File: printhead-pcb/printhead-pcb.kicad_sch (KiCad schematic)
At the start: 22 parts, among them Q1 2N3819, Q2 BSS138, Q3 2N3819, Q4 BSS138, U1 NE555D, U2 NE555D

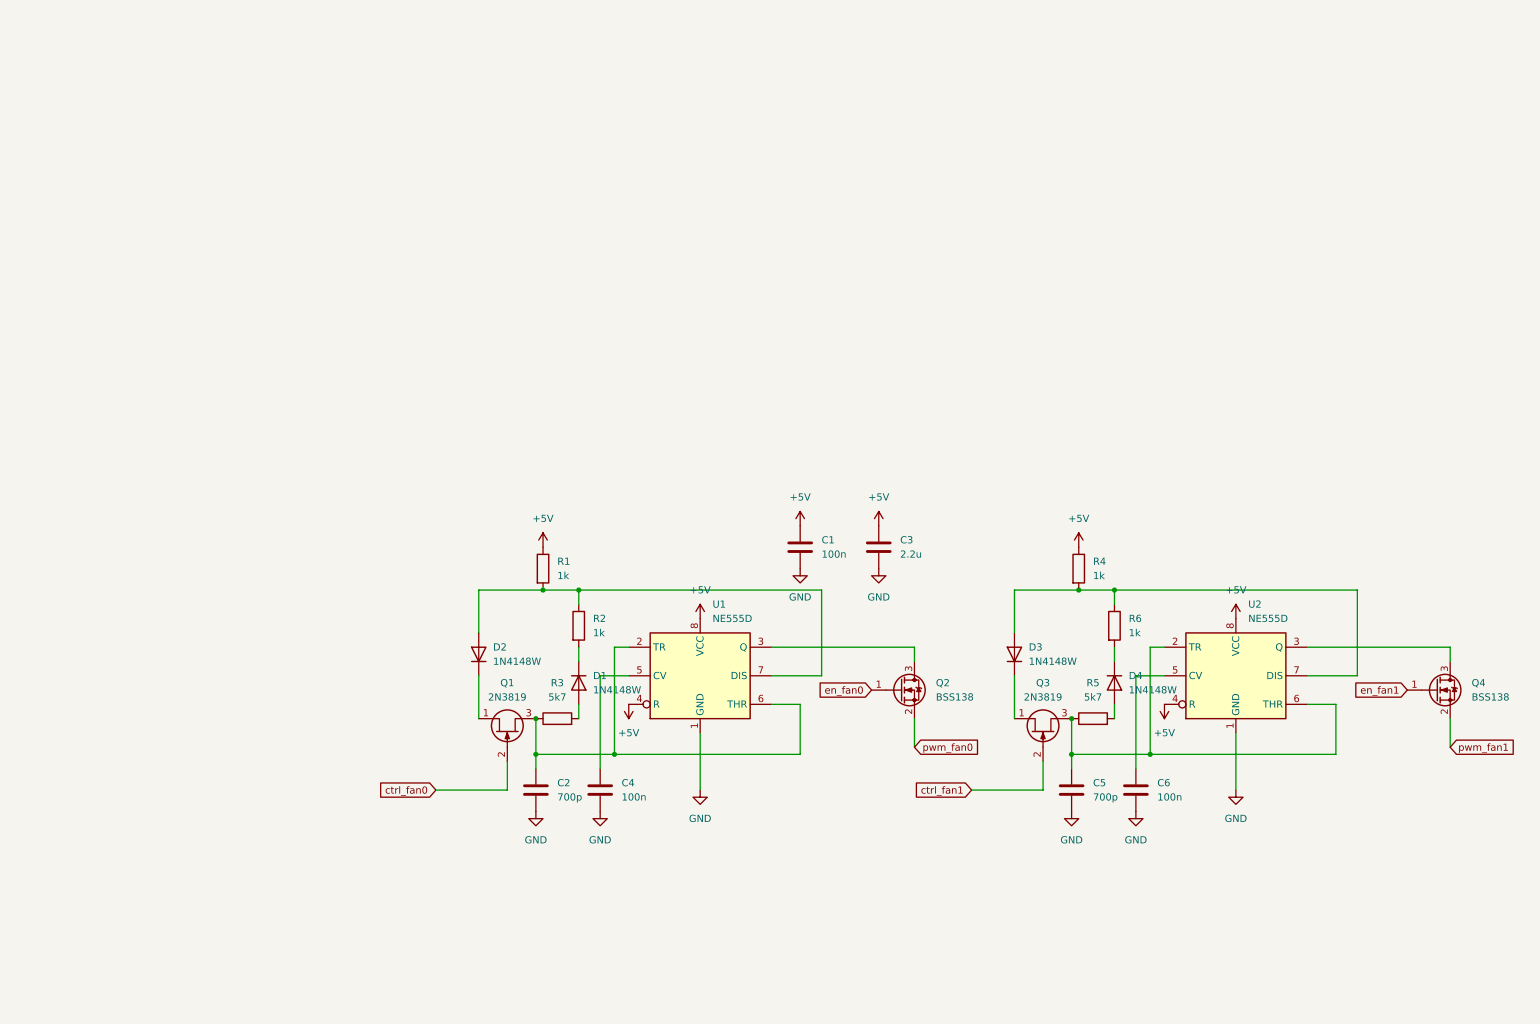
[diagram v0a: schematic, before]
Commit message: power fans, sensors
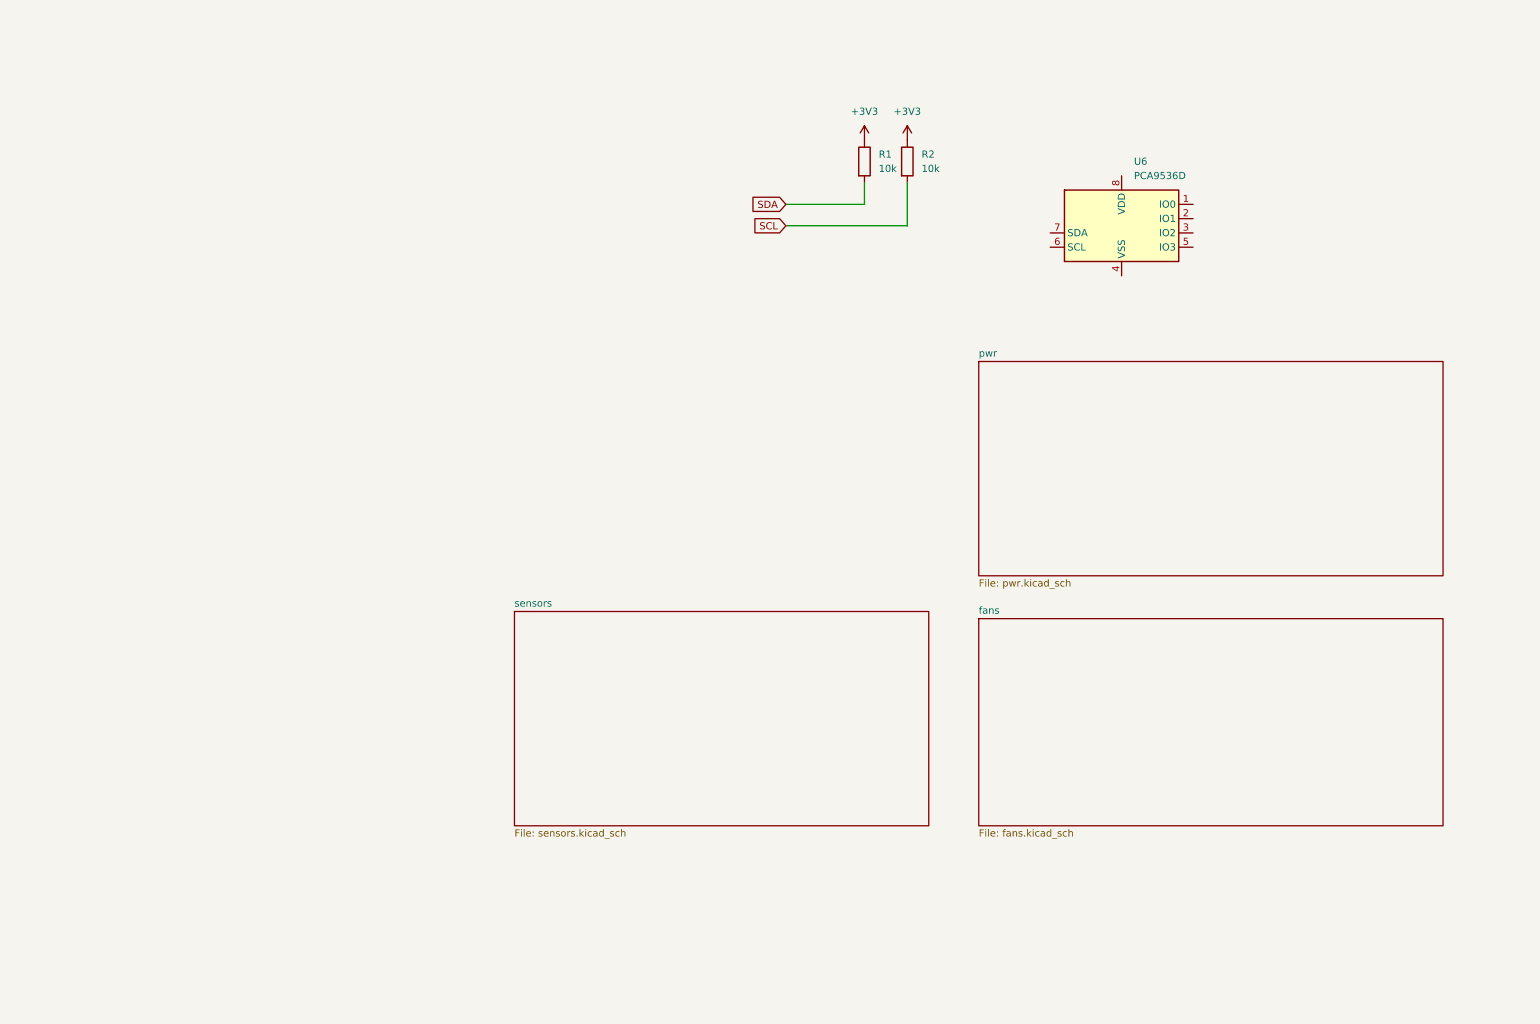
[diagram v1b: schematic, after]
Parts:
- removed C1, C4, C6: 100n, Capacitor_SMD:C_0603_1608Metric, symbol Device:C
- removed C2, C5: 700p, Capacitor_SMD:C_0603_1608Metric, symbol Device:C
- removed C3: 2.2u, Capacitor_SMD:C_1210_3225Metric, symbol Device:C
- removed D1, D2, D3, D4: 1N4148W, Diode_SMD:D_SOD-123, symbol Diode:1N4148W
- removed Q1, Q3: 2N3819, Package_DIP:DIP-8_W7.62mm_SMDSocket_SmallPads, symbol Transistor_FET:2N3819
- removed Q2, Q4: BSS138, Package_TO_SOT_SMD:SOT-23, symbol Transistor_FET:BSS138
- removed R3, R5: 5k7, Resistor_SMD:R_0603_1608Metric, symbol Device:R
- removed R4, R6: 1k, Resistor_SMD:R_0603_1608Metric, symbol Device:R
- removed U1, U2: NE555D, Package_SO:SOIC-8_3.9x4.9mm_P1.27mm, symbol Timer:NE555D
- added U6: PCA9536D, Package_SO:SOIC-8_3.9x4.9mm_P1.27mm, symbol Interface_Expansion:PCA9536D
- R1, R2: value 1k -> 10k; footprint Resistor_SMD:R_0603_1608Metric -> (none)
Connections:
- net +5V is gone; now on net +3V3: R1.1
- net +3V3: now reaches R2.1
- net +3V3: no longer R1.2
- net SCL: now reaches R2.2
- new net SDA: R1.2
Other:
- added sheet fans (fans.kicad_sch)
- added sheet pwr (pwr.kicad_sch)
- added sheet sensors (sensors.kicad_sch)

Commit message: circuit finished?
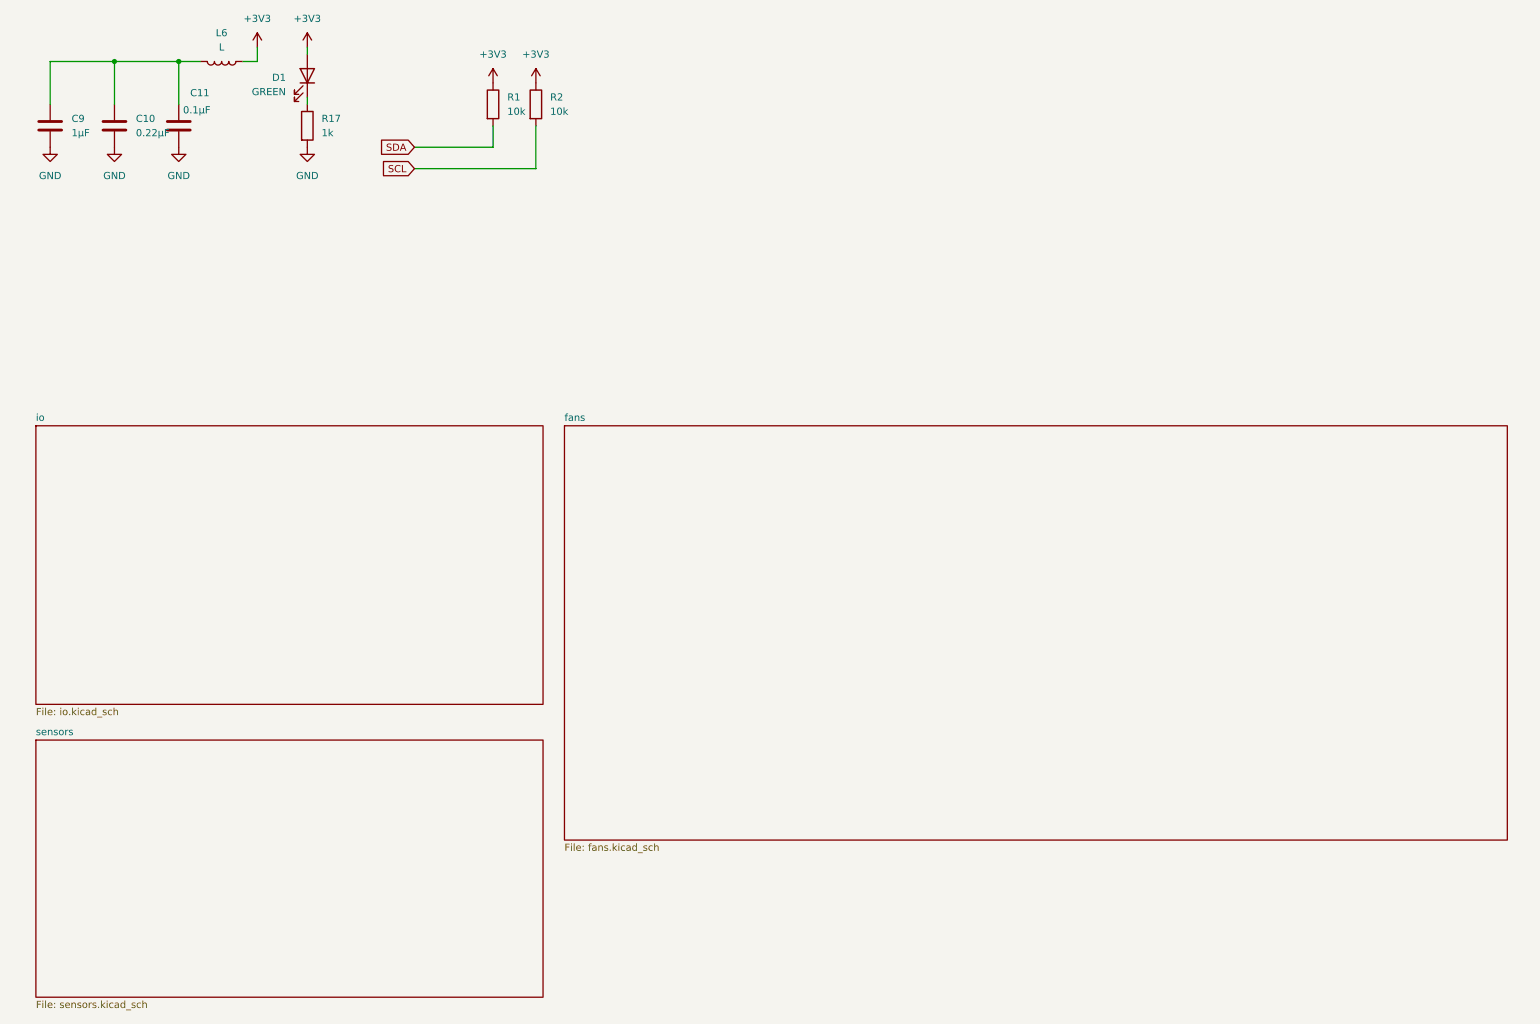
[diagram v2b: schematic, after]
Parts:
- removed U6: PCA9536D, Package_SO:SOIC-8_3.9x4.9mm_P1.27mm, symbol Interface_Expansion:PCA9536D
- added C10: 0.22µF, Capacitor_SMD:C_0402_1005Metric, symbol Device:C
- added C11: 0.1µF, Capacitor_SMD:C_0402_1005Metric, symbol Device:C
- added C9: 1µF, Capacitor_SMD:C_0402_1005Metric, symbol Device:C
- added D1: GREEN, LED_SMD:LED_0805_2012Metric, symbol Device:LED
- added L6: L, Inductor_SMD:L_0402_1005Metric, symbol Device:L
- added R17: 1k, Resistor_SMD:R_0402_1005Metric, symbol Device:R
- R1, R2: footprint (none) -> Resistor_SMD:R_0402_1005Metric
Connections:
- net +3V3: now also D1.2 (A), L6.1
- new net: D1.1 (K), R17.1
- new net: C10.1, C11.1, C9.1, L6.2
- new net GND: C10.2, C11.2, C9.2, R17.2
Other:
- removed sheet pwr
- added sheet io (io.kicad_sch)
- title: (none) -> Printhead PCB
- moved on the sheet: R1, R2

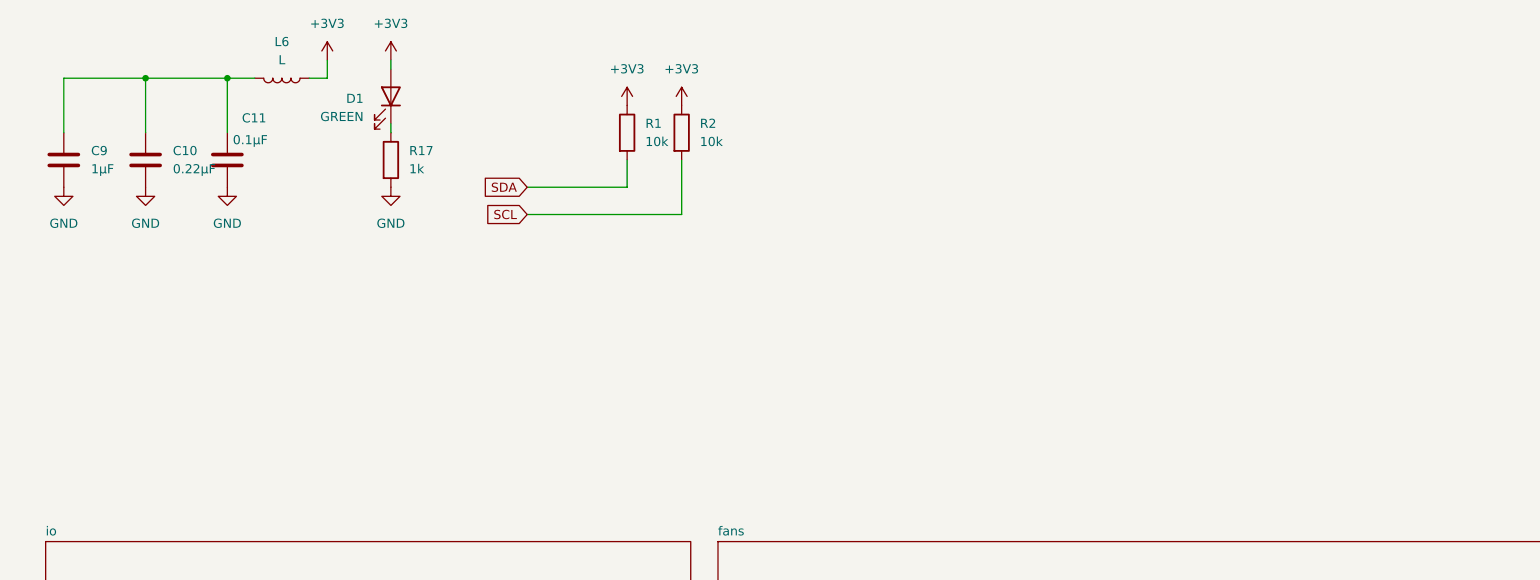
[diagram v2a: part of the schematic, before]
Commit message: layout
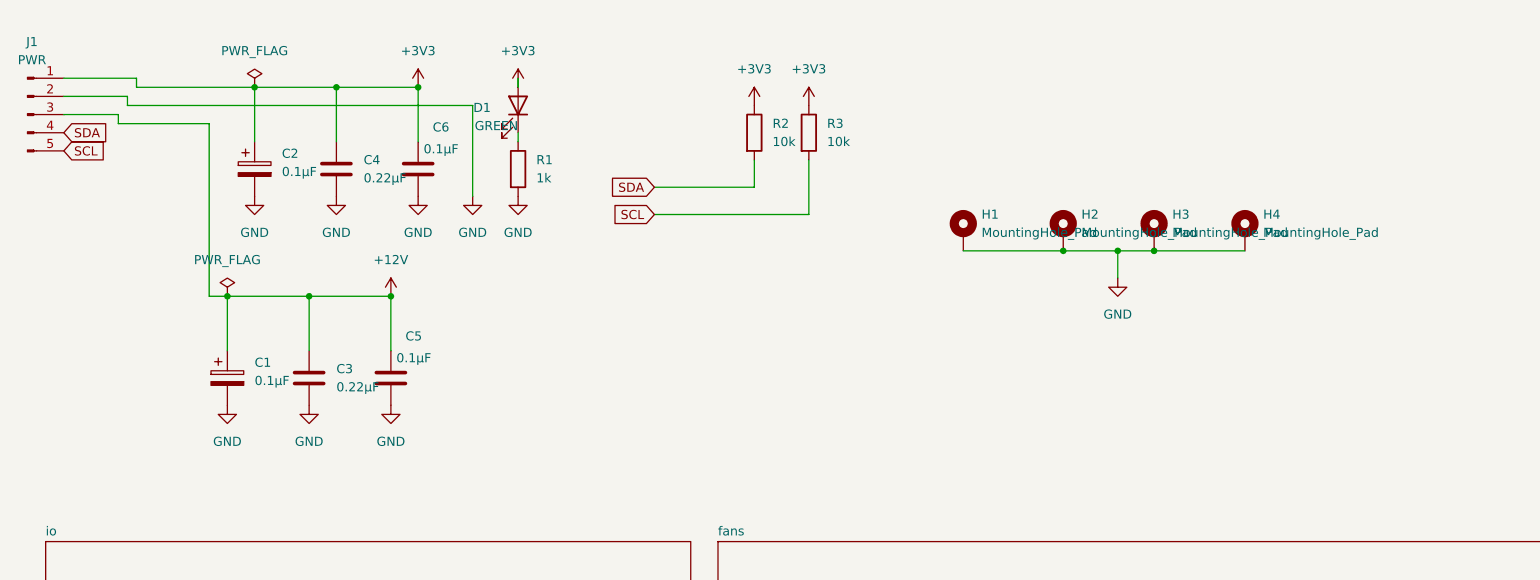
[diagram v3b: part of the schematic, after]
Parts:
- removed C9: 1µF, Capacitor_SMD:C_0402_1005Metric, symbol Device:C
- removed L6: L, Inductor_SMD:L_0402_1005Metric, symbol Device:L
- added C1, C2: 0.1µF, Capacitor_SMD:CP_Elec_5x3, symbol Device:C_Polarized
- added C3: 0.22µF, Capacitor_SMD:C_0402_1005Metric, symbol Device:C
- added C5: 0.1µF, Capacitor_SMD:C_0402_1005Metric, symbol Device:C
- added H1, H2, H3, H4: MountingHole_Pad, MountingHole:MountingHole_2.2mm_M2_Pad_TopBottom, symbol Mechanical:MountingHole_Pad
- added J1: PWR, Connector_JST:JST_EH_S5B-EH_1x05_P2.50mm_Horizontal, symbol Connector:Conn_01x05_Male
- renumbered C10 to C4, C11 to C6, R17 to R1, R1 to R2, R2 to R3
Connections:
- net +3V3: now also C4.1, C6.1, C2.1, J1.1 (Pin_1)
- net GND: now also C1.2, C2.2, C3.2, C5.2, H1.1, H2.1, H3.1, H4.1, J1.2 (Pin_2)
- net SCL: now also J1.5 (Pin_5)
- net SDA: now also J1.4 (Pin_4)
- new net +12V: C1.1, C3.1, C5.1, J1.3 (Pin_3)
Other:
- moved on the sheet: C4, C6, D1, R1, R2, R3
